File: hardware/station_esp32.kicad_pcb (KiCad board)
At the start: 2 copper layers, 50.8 x 40.6 mm, 8 parts, among them J1 Conn_01x04, U1 DHT11, U2 ESP32-WROOM-32

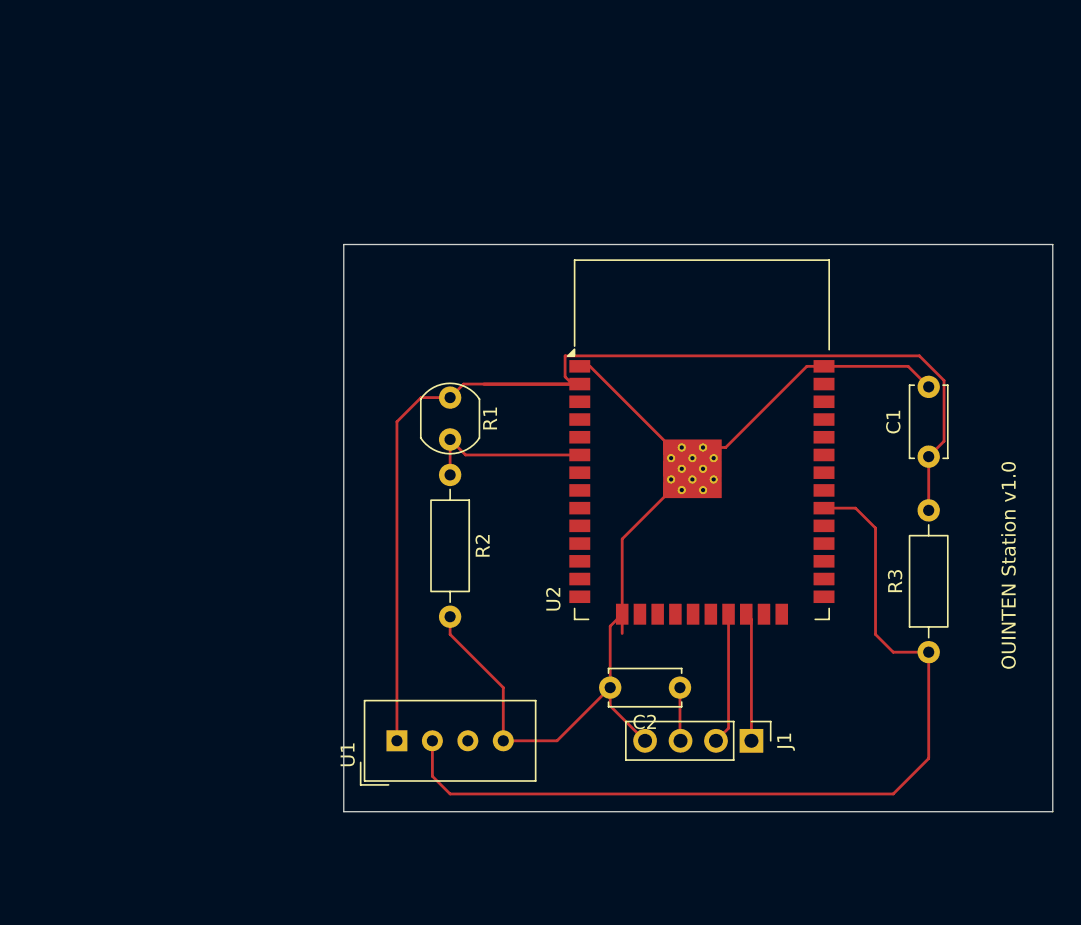
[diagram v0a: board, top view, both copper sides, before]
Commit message: Add files via upload
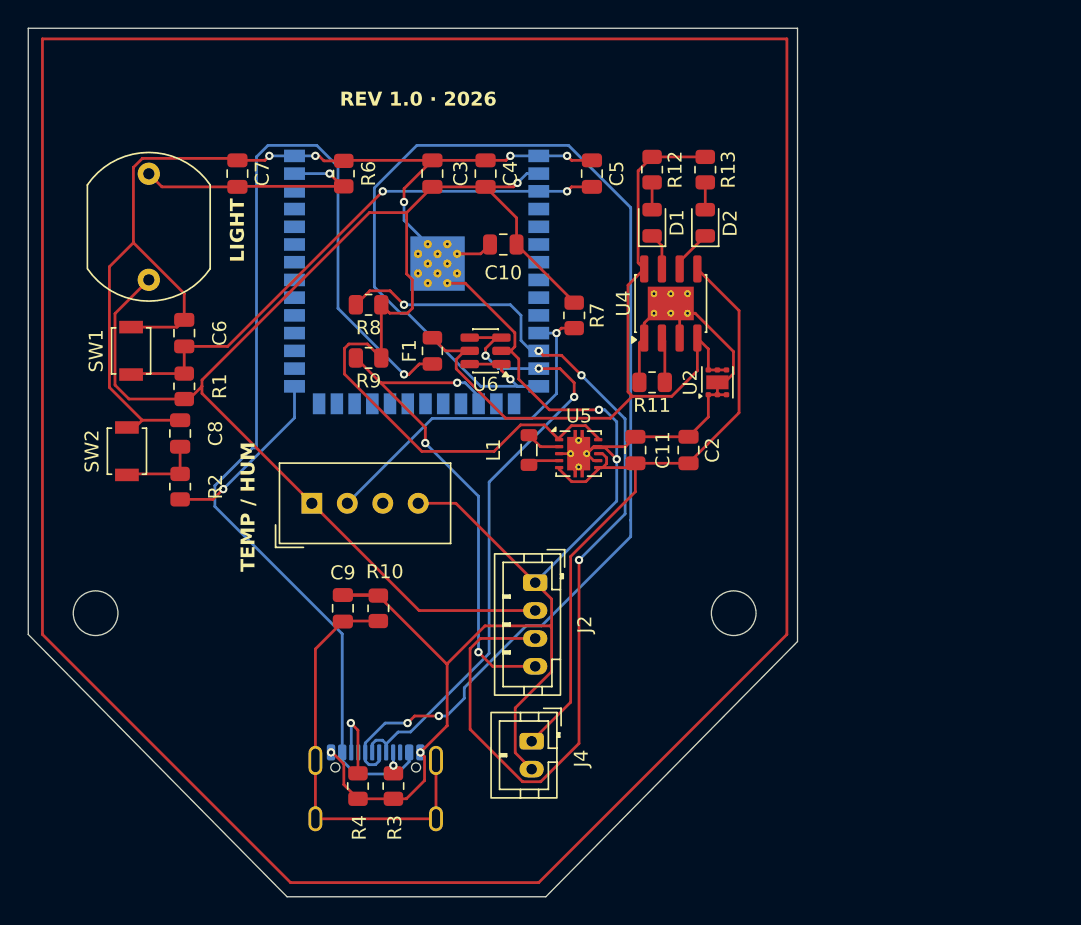
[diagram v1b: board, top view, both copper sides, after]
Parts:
- removed C1: 100nF, Capacitor_THT:C_Disc_D5.0mm_W2.5mm_P5.00mm
- added C10: C, Capacitor_SMD:C_0805_2012Metric, F.Cu at (139.7, 73.7)
- added C11: C, Capacitor_SMD:C_0805_2012Metric, F.Cu at (149.2, 88.4)
- added C3: C, Capacitor_SMD:C_0805_2012Metric, F.Cu at (134.6, 68.6)
- added C4: C, Capacitor_SMD:C_0805_2012Metric, F.Cu at (138.4, 68.6)
- added C5: C, Capacitor_SMD:C_0805_2012Metric, F.Cu at (146.1, 68.6)
- added C6: C, Capacitor_SMD:C_0805_2012Metric, F.Cu at (116.8, 80.0)
- added C7: C, Capacitor_SMD:C_0805_2012Metric, F.Cu at (120.7, 68.6)
- added C8: C, Capacitor_SMD:C_0805_2012Metric, F.Cu at (116.5, 87.2)
- added C9: C, Capacitor_SMD:C_0805_2012Metric, F.Cu at (128.2, 99.7)
- added D1: LED, LED_SMD:LED_0805_2012Metric, F.Cu at (150.4, 72.1)
- added D2: LED, LED_SMD:LED_0805_2012Metric, F.Cu at (154.2, 72.1)
- added F1: Fuse, Fuse:Fuse_0805_2012Metric, F.Cu at (134.6, 81.3)
- added J2: Conn_01x04_Socket, Connector_JST:JST_PH_B4B-PH-K_1x04_P2.00mm_Vertical, F.Cu at (142.0, 97.9)
- added J4: Conn_01x02_Socket, Connector_JST:JST_PH_B2B-PH-K_1x02_P2.00mm_Vertical, F.Cu at (141.7, 109.3)
- added L1: L, Inductor_SMD:L_0805_2012Metric, F.Cu at (141.5, 88.4)
- added R10: R, Resistor_SMD:R_0805_2012Metric, F.Cu at (130.7, 99.7)
- added R11: R, Resistor_SMD:R_0805_2012Metric, F.Cu at (150.4, 83.5)
- added R12: R, Resistor_SMD:R_0805_2012Metric, F.Cu at (150.4, 68.3)
- added R13: R, Resistor_SMD:R_0805_2012Metric, F.Cu at (154.2, 68.3)
- added R4: R, Resistor_SMD:R_0805_2012Metric, F.Cu at (129.3, 112.5)
- added R5: LDR03, OptoDevice:R_LDR_10x8.5mm_P7.6mm_Vertical, F.Cu at (114.3, 76.2)
- added R6: R, Resistor_SMD:R_0805_2012Metric, F.Cu at (128.3, 68.6)
- added R7: R, Resistor_SMD:R_0805_2012Metric, F.Cu at (144.8, 78.7)
- added R8: R, Resistor_SMD:R_0805_2012Metric, F.Cu at (130.0, 78.0)
- added R9: R, Resistor_SMD:R_0805_2012Metric, F.Cu at (130.0, 81.8)
- added REF**: MountingHole_3.2mm_M3, MountingHole:MountingHole_3.2mm_M3, F.Cu at (110.5, 100.1)
- added REF**: MountingHole_3.2mm_M3, MountingHole:MountingHole_3.2mm_M3, F.Cu at (156.2, 100.1)
- added SW1: SW_SPST, Button_Switch_SMD:SW_SPST_B3U-1000P, F.Cu at (113.0, 81.3)
- added SW2: SW_SPST, Button_Switch_SMD:SW_SPST_B3U-1000P, F.Cu at (112.7, 88.5)
- added U3: DHT11, Sensor:Aosong_DHT11_5.5x12.0_P2.54mm, F.Cu at (126.0, 92.2)
- added U4: TP4056-42-ESOP8, Package_SO:SOIC-8-1EP_3.9x4.9mm_P1.27mm_EP2.41x3.3mm_ThermalVias, F.Cu at (151.7, 77.9)
- added U5: TPS63001, Package_SON:Texas_DRC0010J_ThermalVias, F.Cu at (145.1, 88.6)
- added U6: USBLC6-2SC6, Package_TO_SOT_SMD:SOT-23-6, F.Cu at (138.4, 81.3)
- C2: value 100nF -> C; footprint Capacitor_THT:C_Disc_D5.0mm_W2.5mm_P5.00mm -> Capacitor_SMD:C_0805_2012Metric
- J1: value Conn_01x04 -> USB_C_Receptacle_USB2.0_16P; footprint Connector_PinHeader_2.54mm:PinHeader_1x04_P2.54mm_Vertical -> Connector_USB:USB_C_Receptacle_GCT_USB4105-xx-A_16P_TopMnt_Horizontal; moved to B.Cu
- R1: value R_Photo -> R; footprint OptoDevice:R_LDR_5.0x4.1mm_P3mm_Vertical -> Resistor_SMD:R_0805_2012Metric
- R2, R3: value 10k -> R; footprint Resistor_THT:R_Axial_DIN0207_L6.3mm_D2.5mm_P10.16mm_Horizontal -> Resistor_SMD:R_0805_2012Metric
- U1: value DHT11 -> ESP32-S3-WROOM-1; footprint Sensor:Aosong_DHT11_5.5x12.0_P2.54mm -> RF_Module:ESP32-S3-WROOM-1; moved to B.Cu
- U2: value ESP32-WROOM-32 -> TVS0500DRV; footprint RF_Module:ESP32-WROOM-32 -> Package_SON:WSON-6-1EP_2x2mm_P0.65mm_EP1x1.6mm
- moved R3 39.5 mm to (131.8, 112.5), turned to -90 degrees
- moved U1 36.7 mm to (133.5, 72.6), turned to 180 degrees
- moved J1 27.3 mm to (130.6, 113.7), turned to 180 degrees
- moved R2 19.4 mm to (116.5, 91.0), turned to 90 degrees
- moved R1 19.1 mm to (116.8, 83.8), turned to 90 degrees
- moved C2 17.0 mm to (153.0, 88.4), turned to 90 degrees
- moved U2 7.19 mm to (155.0, 83.5), turned to 90 degrees
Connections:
- C2 pad 1: +5V -> BAT
- R1 pad 1: +3.3V -> +3V3
- R1 pad 2: Net-(U2-IO34) -> EN
- R2 pad 1: Net-(U2-IO34) -> BOOT
- R2 pad 2: GND -> Net-(SW2-A)
- R3 pad 1: Net-(U1-DATA) -> Net-(J1-CC1)
- R3 pad 2: +3.3V -> GND
- U1 pad 1: +3.3V -> GND
- U1 pad 2: Net-(U1-DATA) -> +3V3
- U1 pad 3: unconnected-(U1-NC-Pad3) -> EN
- U1 pad 4: GND -> unconnected-(U1-IO4-Pad4)
- U2 pad 2: +3.3V -> GND
- U2 pad 3: unconnected-(U2-EN-Pad3) -> GND
- U2 pad 4: unconnected-(U2-SENSOR_VP-Pad4) -> VBUS
- U2 pad 5: unconnected-(U2-SENSOR_VN-Pad5) -> VBUS
- U2 pad 6: Net-(U2-IO34) -> VBUS
- U2 pad 7: unconnected-(U2-IO35-Pad7) -> GND
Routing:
- net GND: track 69.3 -> 212.1 mm, vias 0 -> 9
- net +3V3: track 0.00 -> 129.3 mm, vias 0 -> 1
- net D+: track 0.00 -> 101.4 mm, vias 0 -> 3
- net +3.3V: track 84.4 -> 0.00 mm
- net VBUS_IN: track 0.00 -> 80.7 mm, vias 0 -> 1
- net SDA: track 0.00 -> 70.4 mm, vias 0 -> 4
- net Net-(U1-DATA): track 63.5 -> 0.00 mm
- net VBUS: track 0.00 -> 53.5 mm
- net BAT: track 0.00 -> 51.9 mm
- net D-: track 0.00 -> 45.8 mm, vias 0 -> 3
- net EN: track 0.00 -> 39.7 mm, vias 0 -> 2
- net SCL: track 0.00 -> 37.2 mm, vias 0 -> 3
- net Net-(J1-SHIELD): track 0.00 -> 30.6 mm
- net DHT_DATA: track 0.00 -> 25.8 mm, vias 0 -> 1
- net LUMINOSITE: track 0.00 -> 18.3 mm, vias 0 -> 1
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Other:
- board size 50.8 x 40.6 mm -> 55.1 x 62.2 mm
- board text added: "5V USB"
- board text added: "DESIGNED IN GRENOBLE"
- board text added: "ENVIRONMENTAL STATION"
- board text added: "LIGHT"
- board text added: "REV 1.0 · 2026"
- board text added: "TEMP / HUM"
- board text removed: "OUINTEN Station v1.0"
